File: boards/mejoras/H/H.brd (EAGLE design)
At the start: 100 x 45 mm, 3 parts, among them IC1 PIC18F4550_TQFP

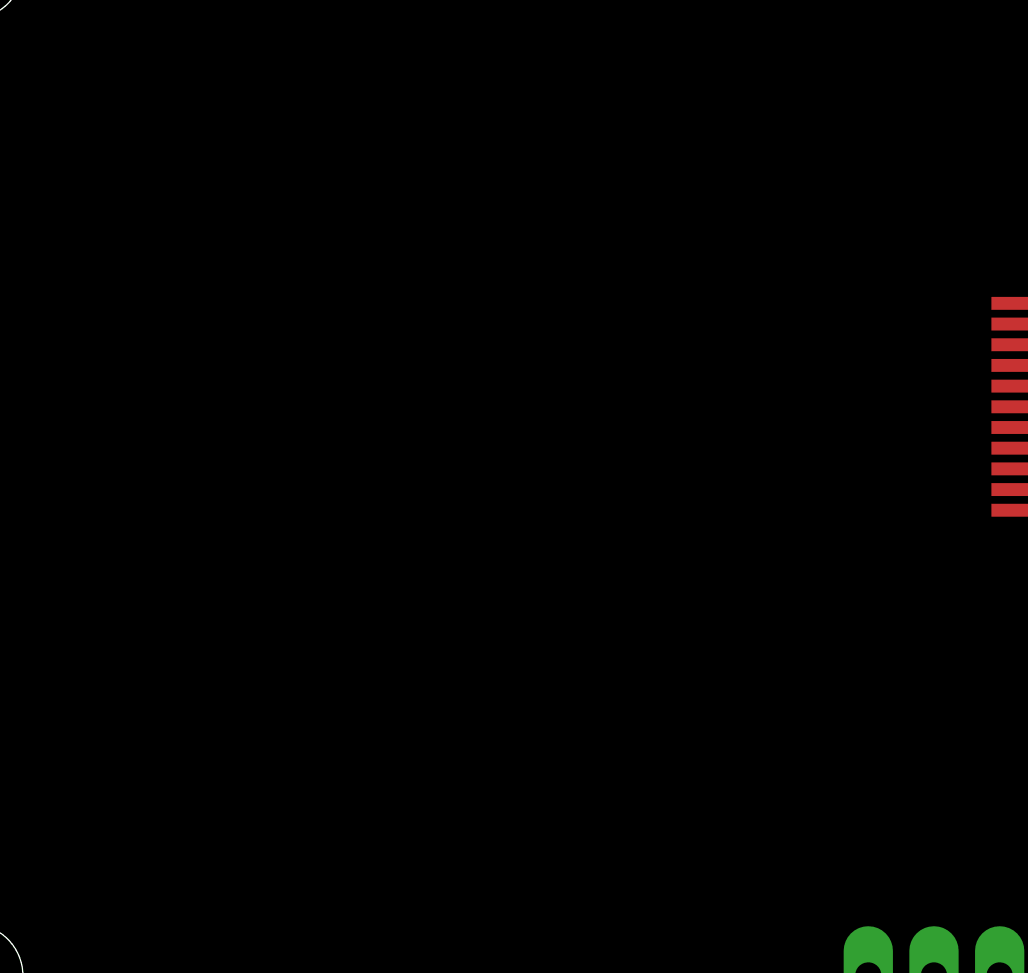
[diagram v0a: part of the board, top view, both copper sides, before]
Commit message: changes to g circuit
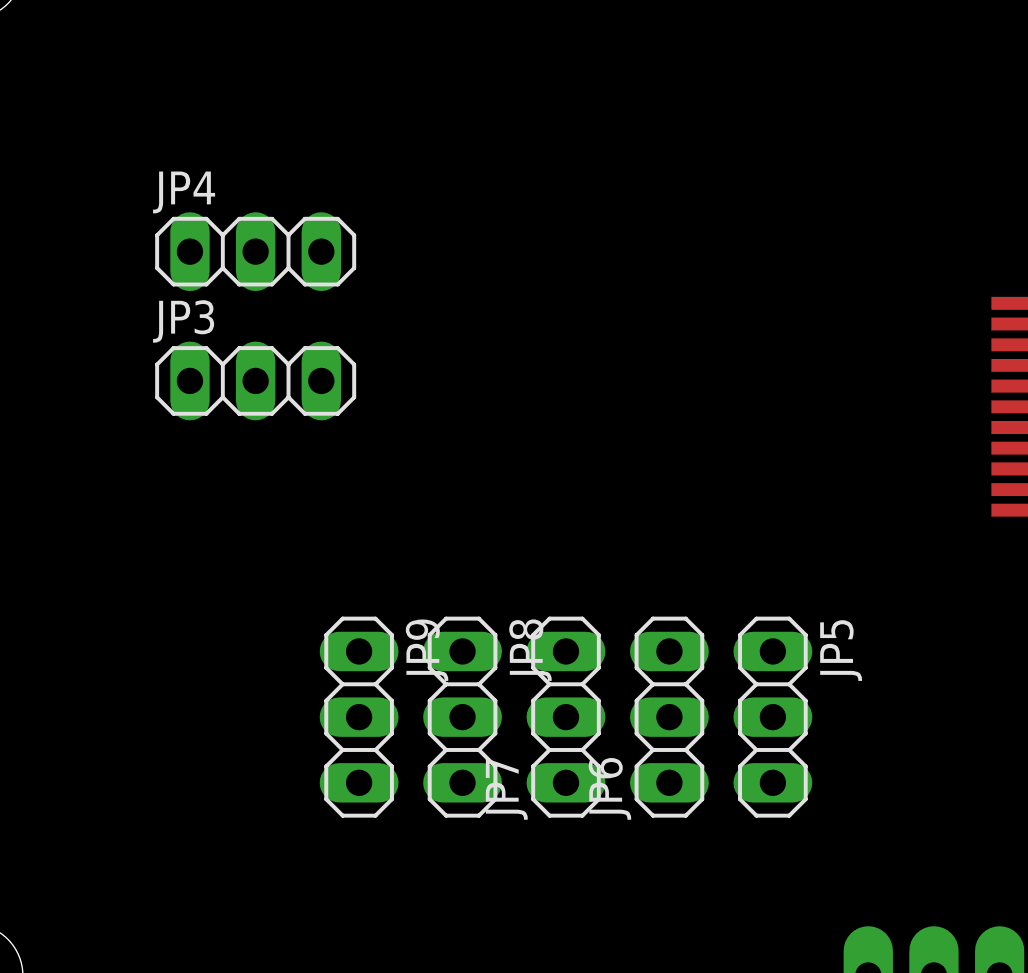
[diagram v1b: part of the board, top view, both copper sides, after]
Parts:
- added JP3, JP4, JP5, JP6, JP7, JP8, JP9: (no value), pinhead:1X03
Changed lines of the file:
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@@
 <?xml version="1.0" encoding="utf-8"?>
 <!DOCTYPE eagle SYSTEM "eagle.dtd">
-<eagle version="9.6.2">
+<eagle version="9.6.0">
 <drawing>
 <settings>
@@
 <attribute name="VALUE" x="45.936" y="23.2299" size="1.778" layer="27"/>
 </element>
+<element name="JP3" library="pinhead" library_urn="urn:adsk.eagle:library:325" package="1X03" package3d_urn="urn:adsk.eagle:package:22458/2" value="" x="15" y="26" smashed="yes">
+<attribute name="NAME" x="11.1138" y="27.8288" size="1.27" layer="25" ratio="10"/>
+<attribute name="POPULARITY" value="92" x="15" y="26" size="1.778" layer="27" display="off"/>
+<attribute name="VALUE" x="11.19" y="22.825" size="1.27" layer="27"/>
+</element>
+<element name="JP4" library="pinhead" library_urn="urn:adsk.eagle:library:325" package="1X03" package3d_urn="urn:adsk.eagle:package:22458/2" value="" x="15" y="31" smashed="yes">
+<attribute name="NAME" x="11.1138" y="32.8288" size="1.27" layer="25" ratio="10"/>
+<attribute name="POPULARITY" value="92" x="15" y="31" size="1.778" layer="27" display="off"/>
+<attribute name="VALUE" x="11.19" y="27.825" size="1.27" layer="27"/>
+</element>
+<element name="JP5" library="pinhead" library_urn="urn:adsk.eagle:library:325" package="1X03" package3d_urn="urn:adsk.eagle:package:22458/2" value="" x="35" y="13" smashed="yes" rot="R270">
+<attribute name="NAME" x="36.8288" y="16.8862" size="1.27" layer="25" ratio="10" rot="R270"/>
+<attribute name="POPULARITY" value="92" x="35" y="13" size="1.778" layer="27" rot="R270" display="off"/>
+<attribute name="VALUE" x="31.825" y="16.81" size="1.27" layer="27" rot="R270"/>
+</element>
+<element name="JP6" library="pinhead" library_urn="urn:adsk.eagle:library:325" package="1X03" package3d_urn="urn:adsk.eagle:package:22458/2" value="" x="31" y="13" smashed="yes" rot="R90">
+<attribute name="NAME" x="29.1712" y="9.1138" size="1.27" layer="25" ratio="10" rot="R90"/>
+<attribute name="POPULARITY" value="92" x="31" y="13" size="1.778" layer="27" rot="R90" display="off"/>
+<attribute name="VALUE" x="34.175" y="9.19" size="1.27" layer="27" rot="R90"/>
+</element>
+<element name="JP7" library="pinhead" library_urn="urn:adsk.eagle:library:325" package="1X03" package3d_urn="urn:adsk.eagle:package:22458/2" value="" x="27" y="13" smashed="yes" rot="R90">
+<attribute name="NAME" x="25.1712" y="9.1138" size="1.27" layer="25" ratio="10" rot="R90"/>
+<attribute name="POPULARITY" value="92" x="27" y="13" size="1.778" layer="27" rot="R90" display="off"/>
+<attribute name="VALUE" x="30.175" y="9.19" size="1.27" layer="27" rot="R90"/>
+</element>
+<element name="JP8" library="pinhead" library_urn="urn:adsk.eagle:library:325" package="1X03" package3d_urn="urn:adsk.eagle:package:22458/2" value="" x="23" y="13" smashed="yes" rot="R270">
+<attribute name="NAME" x="24.8288" y="16.8862" size="1.27" layer="25" ratio="10" rot="R270"/>
+<attribute name="POPULARITY" value="92" x="23" y="13" size="1.778" layer="27" rot="R270" display="off"/>
+<attribute name="VALUE" x="19.825" y="16.81" size="1.27" layer="27" rot="R270"/>
+</element>
+<element name="JP9" library="pinhead" library_urn="urn:adsk.eagle:library:325" package="1X03" package3d_urn="urn:adsk.eagle:package:22458/2" value="" x="19" y="13" smashed="yes" rot="R270">
+<attribute name="NAME" x="20.8288" y="16.8862" size="1.27" layer="25" ratio="10" rot="R270"/>
+<attribute name="POPULARITY" value="92" x="19" y="13" size="1.778" layer="27" rot="R270" display="off"/>
+<attribute name="VALUE" x="15.825" y="16.81" size="1.27" layer="27" rot="R270"/>
+</element>
 </elements>

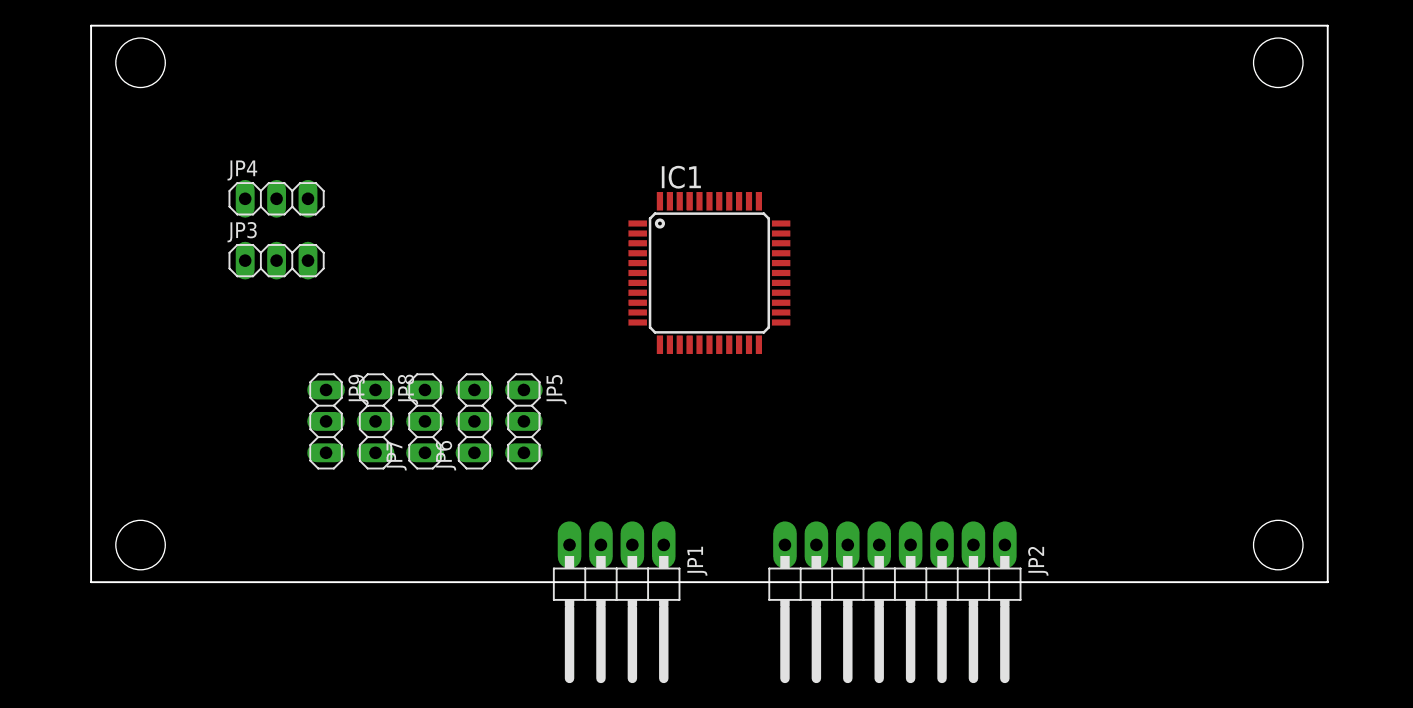
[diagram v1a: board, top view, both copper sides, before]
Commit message: udpated new circuits
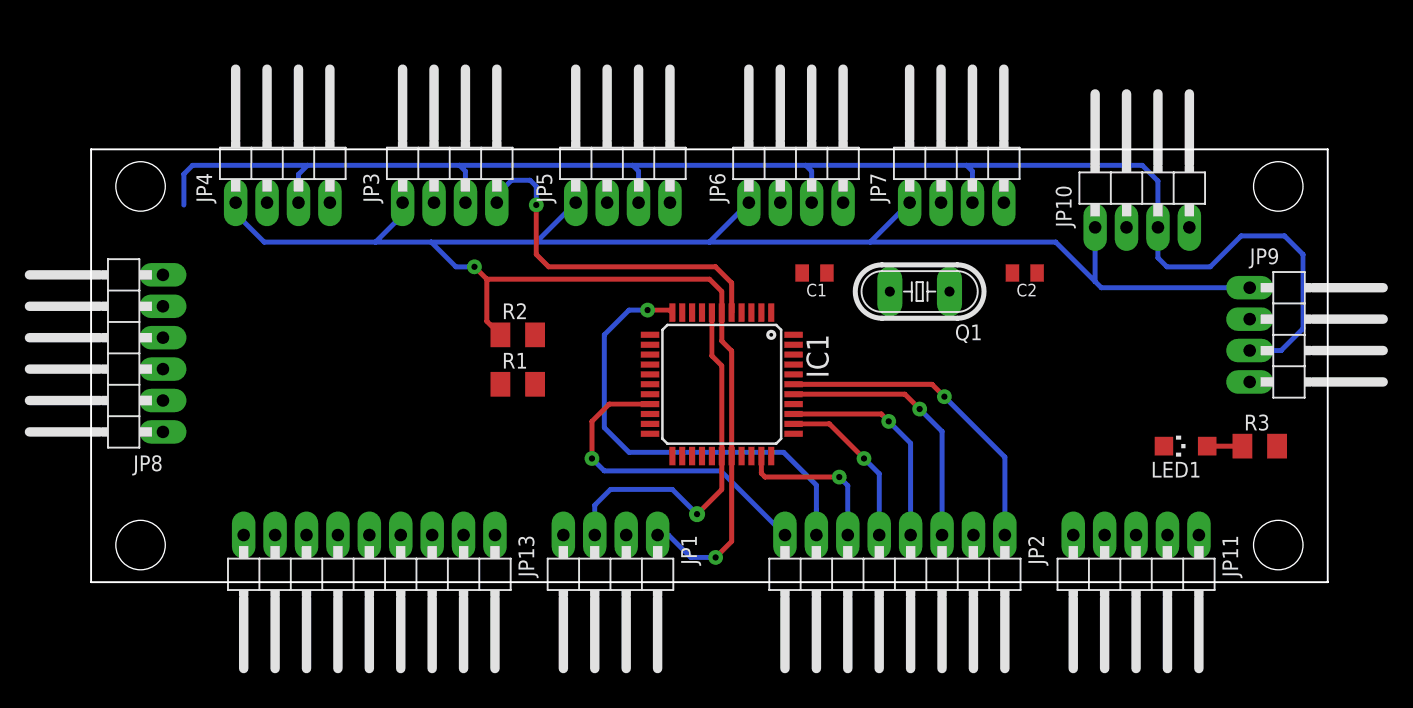
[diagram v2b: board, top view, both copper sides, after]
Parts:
- added C1, C2: (no value), adafruit:C0805K
- added JP10: (no value), pinhead-enhanced:1X04/90
- added JP11: (no value), pinhead-enhanced-3:1X05/90
- added JP13: (no value), pinhead-enhanced-3:1X09/90
- added LED1: (no value), adafruit:CHIPLED_1206
- added Q1: (no value), crystal:HC49/S
- added R1, R2: 10k, adafruit:M1206
- added R3: 220, adafruit:M1206
- IC1: value PIC18F4550_TQFP -> PIC18F4455_TQFP
- JP3, JP4, JP5, JP6, JP7, JP9: device pinhead:1X03 -> pinhead-enhanced:1X04/90
- JP8: device pinhead:1X03 -> pinhead-enhanced-2:1X06/90
- moved JP9 78.8 mm to (97.5, 20.0)
- moved JP7 48.1 mm to (70.0, 34.5), turned to 0 degrees
- moved JP6 33.7 mm to (57.0, 34.5), turned to 0 degrees
- moved JP5 22.9 mm to (43.0, 34.5), turned to 0 degrees
- moved JP8 21.7 mm to (2.00, 18.5), turned to 90 degrees
- moved JP3 16.4 mm to (29.0, 34.5)
- moved IC1 9.06 mm to (51.0, 16.0), turned to 270 degrees
- moved JP4 3.54 mm to (15.5, 34.5)
- moved JP1 0.94 mm to (42.0, 0.00)
- moved JP2 0.80 mm to (65.0, 0.00)
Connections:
- removed net VDD: IC1.28, IC1.7
- removed net VSS: IC1.29, IC1.6
- new net 5V: IC1.28, IC1.7, JP1.3, JP10.3, JP11.1, JP3.3, JP4.3, JP5.3, JP6.3, JP7.3, JP8.3, JP9.3, R3.2
- new net B1: JP13.1
- new net B2: JP13.3
- new net CNY1: IC1.20, JP9.4
- new net CNY2: IC1.21, JP10.4
- new net GND: C1.2, C2.2, IC1.29, IC1.6, JP1.1, JP10.1, JP11.3, JP3.1, JP4.1, JP5.1, JP6.1, JP7.1, JP8.1, JP9.1, LED1.C, R1.1, R2.1
- new net IN1A: IC1.39, JP2.1
- new net IN1B: IC1.38, JP2.3
- new net IN2A: IC1.35, JP2.5
- new net IN2B: IC1.32, JP2.6
- new net LED1: JP13.5
- new net LED2: JP13.6
- new net LED3: JP13.7
- new net LED4: JP13.8
- new net LED5: JP13.9
- new net MCRL: IC1.18, JP8.4
- new net N$1: C1.1, IC1.31, Q1.2
- new net N$2: C2.1, IC1.30, Q1.1
- new net N$3: LED1.A, R3.1
- new net PGC: IC1.16, JP8.6
- new net PGD: IC1.17, JP8.5
- new net POT: JP13.4
- new net PWM1: IC1.36, JP2.4, R1.2
- new net PWM2: IC1.11, JP2.7, R2.2
- new net RX: IC1.1, JP11.4
- new net S1: IC1.5, JP3.4
- new net S2: JP4.4
- new net S3: JP5.4
- new net S4: JP6.4
- new net S5: JP7.4
- new net TX: IC1.44, JP11.5
- new net VPOWER_SENSE: IC1.19, JP2.8
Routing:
- net GND: track 0.00 -> 165.3 mm, vias 0 -> 2
- net 5V: track 0.00 -> 158.7 mm, vias 0 -> 1
- net PWM2: track 0.00 -> 39.1 mm, vias 0 -> 1
- net S1: track 0.00 -> 29.2 mm, vias 0 -> 1
- net VPOWER_SENSE: track 0.00 -> 26.5 mm, vias 0 -> 1
- net IN1A: track 0.00 -> 26.1 mm, vias 0 -> 1
- net IN1B: track 0.00 -> 21.6 mm, vias 0 -> 1
- net PWM1: track 0.00 -> 17.9 mm, vias 0 -> 1
- net IN2A: track 0.00 -> 13.6 mm, vias 0 -> 1
- net IN2B: track 0.00 -> 12.8 mm, vias 0 -> 1
- net N$3: track 0.00 -> 2.85 mm
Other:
- board size 100 x 45 mm -> 100 x 35 mm
